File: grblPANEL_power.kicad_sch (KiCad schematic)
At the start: 24 parts, among them J101 Conn_01x02, U101 MAX17612A, U102 AZ1117-3.3

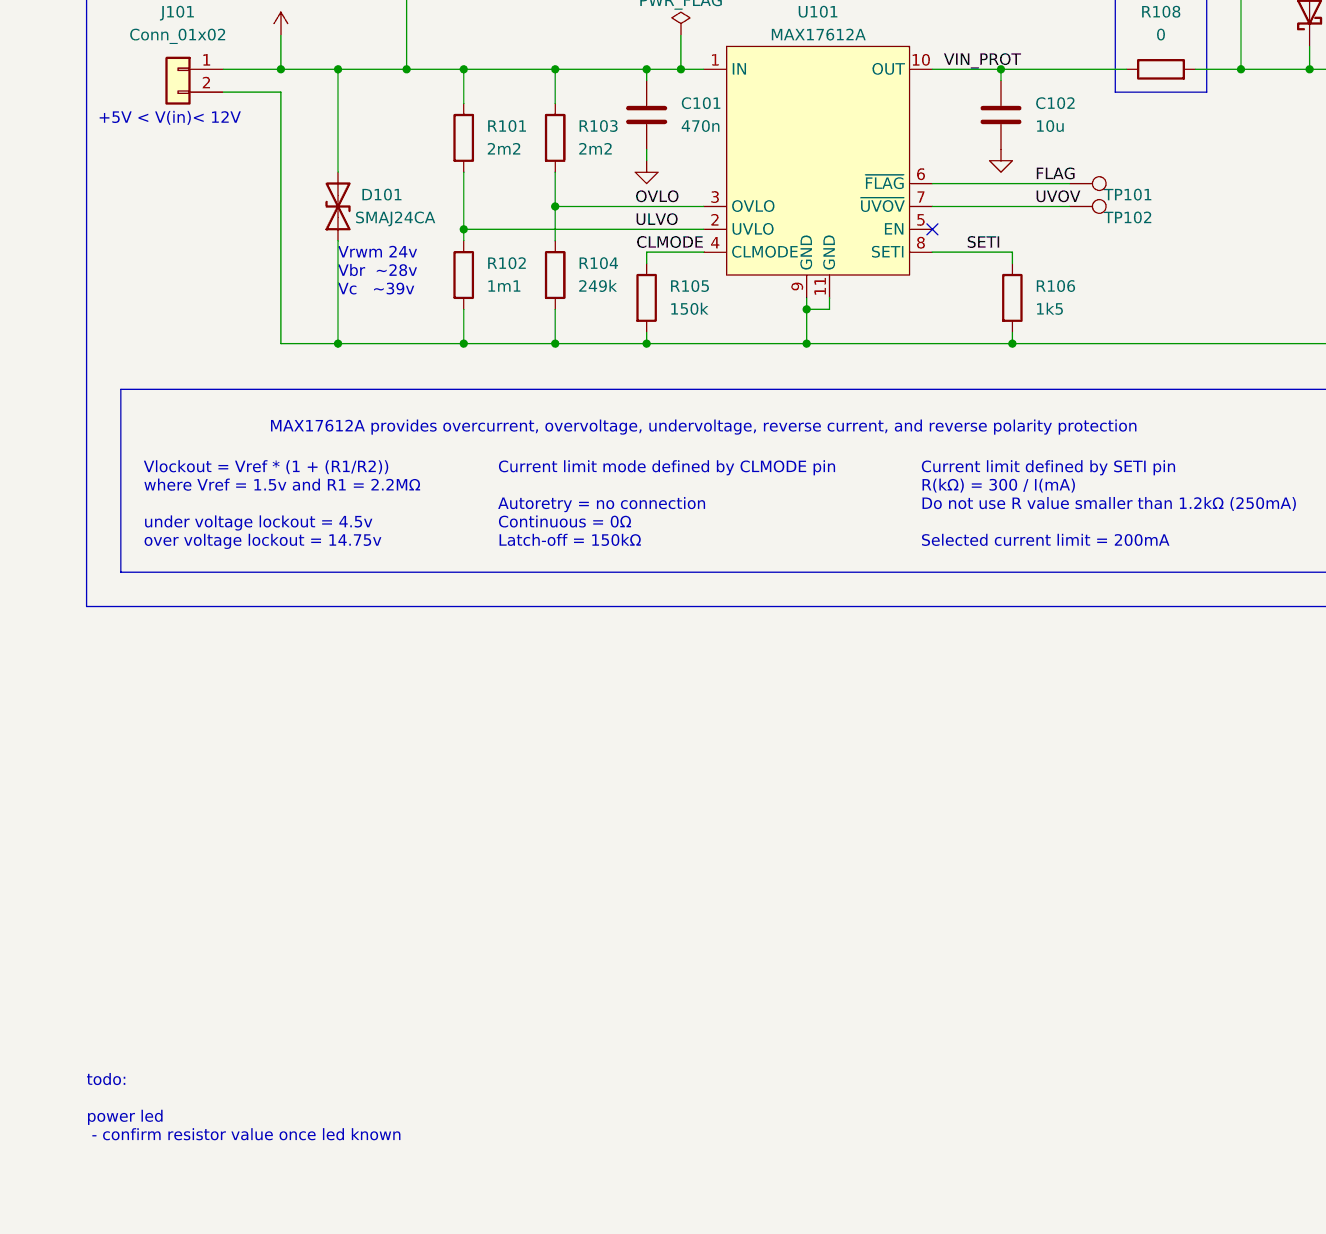
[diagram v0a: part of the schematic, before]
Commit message: Power protection status LEDs - wip
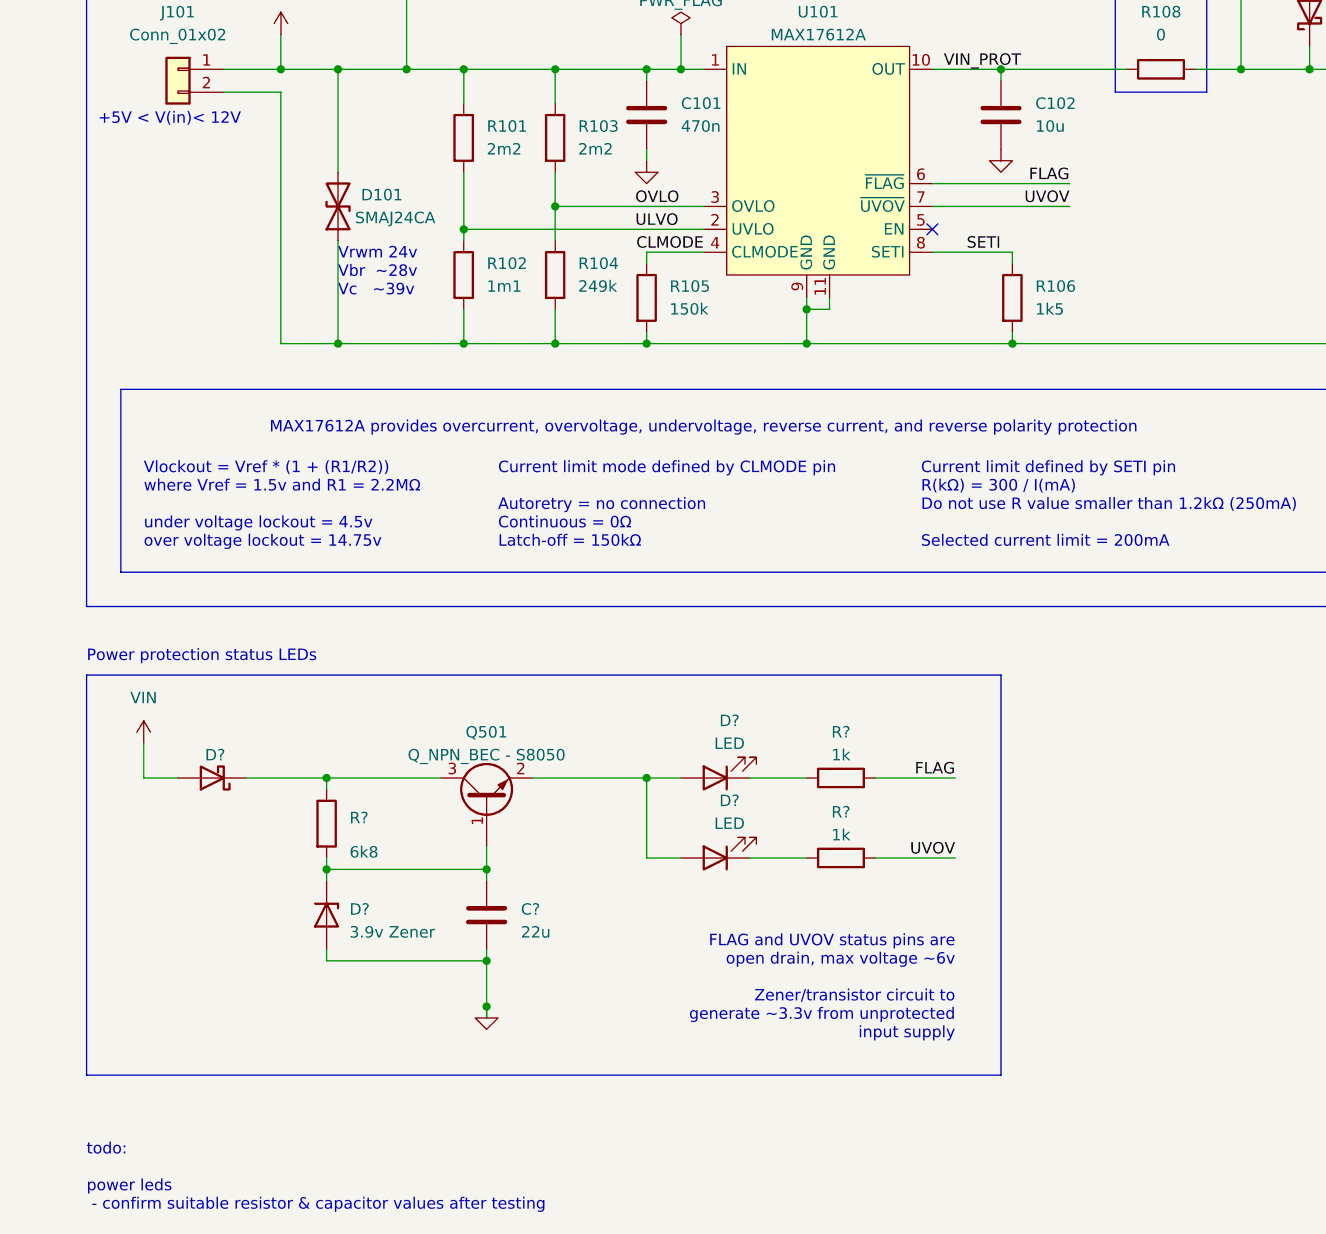
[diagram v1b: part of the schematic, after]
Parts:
- removed TP101, TP102: TestPoint, TestPoint:TestPoint_THTPad_D2.0mm_Drill1.0mm, symbol Connector:TestPoint
- added C?: 22u, Capacitor_SMD:C_0805_2012Metric, symbol Device:C
- added D?: 3.9v Zener, symbol Device:D_Zener
- added D?: D_Schottky, Diode_SMD:D_SOD-323, symbol Device:D_Schottky
- added D? (x2): LED, LED_SMD:LED_0603_1608Metric, symbol Device:LED
- added Q501: Q_NPN_BEC - S8050, Package_TO_SOT_SMD:SOT-23, symbol Device:Q_NPN_BEC
- added R? (x2): 1k, Resistor_SMD:R_0603_1608Metric, symbol Device:R
- added R?: 6k8, Resistor_SMD:R_0603_1608Metric, symbol Device:R
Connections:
- net FLAG: now also R?.2
- net GND: now also C?.2, D?.2 (A)
- net UVOV: now also R?.2
- net VIN: now also D?.2 (A)
- new net: C?.1, D?.1 (K), Q501.1 (B), R?.2
- new net: D?.2 (A), D?.2 (A), Q501.2 (E)
- new net: D?.1 (K), Q501.3 (C), R?.1
- new net: D?.1 (K), R?.1 (x2)
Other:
- note added: "FLAG and UVOV status pins are open drain, max voltage ~6v Zener/transistor circuit to generate ~3.3v from unprotected input supply"
- note added: "Power protection status LEDs"
- note added: "todo: power leds - confirm suitable resistor & capacitor values after testing"
- note removed: "todo: power led - confirm resistor value once led known"
